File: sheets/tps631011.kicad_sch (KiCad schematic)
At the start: 4 parts, among them U2 XC6220B331ER-G

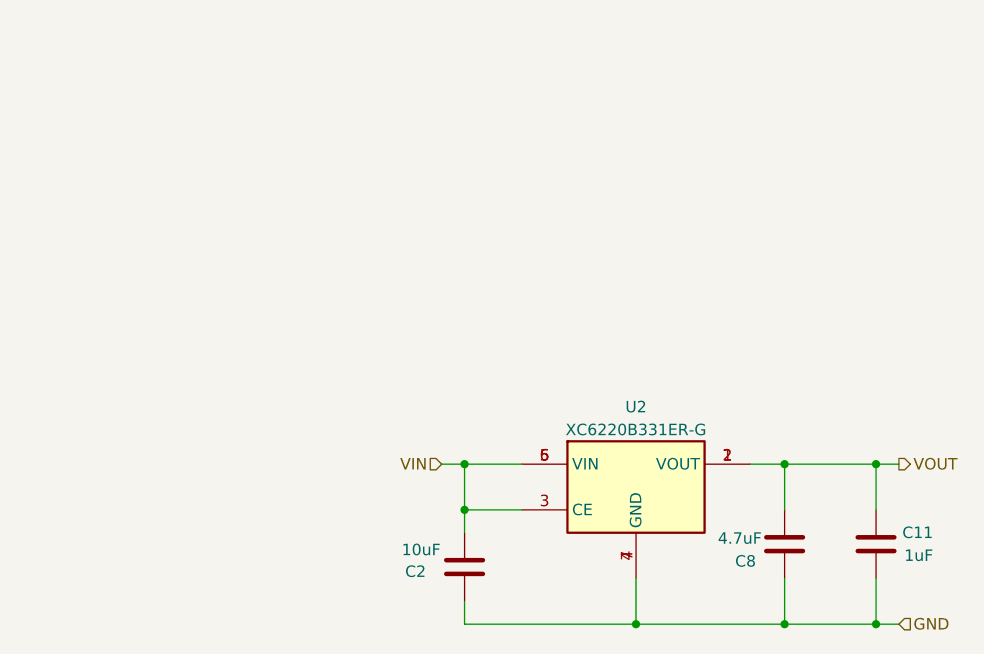
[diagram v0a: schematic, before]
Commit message: More cleanup
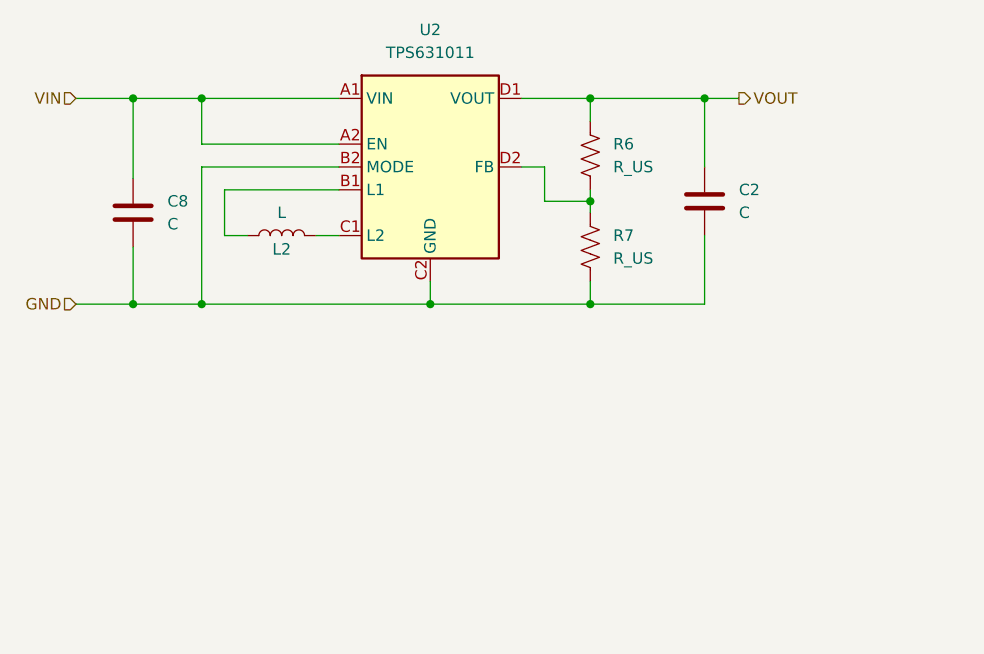
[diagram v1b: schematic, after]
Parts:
- removed C11: 1uF, Capacitor_SMD:C_0402_1005Metric, symbol Device:C
- removed U2: XC6220B331ER-G, PowerFeather:USP-6C_TOR, symbol Regulator_Linear:XC6220B331MR
- added L2: L, symbol Device:L
- added R6, R7: R_US, symbol Device:R_US
- added U2: TPS631011, symbol PowerFeather_KiCAD_Lib:TPS631011
- C2: value 10uF -> C; footprint Capacitor_SMD:C_0603_1608Metric -> (none); Comment 10V, X5R -> (none); MPN 187-CL10A106KP8NNWC -> (none)
- C8: value 4.7uF -> C; footprint Capacitor_SMD:C_0603_1608Metric -> (none); Comment 10V, X5R -> (none); MPN 187-CL10A475KP8NNND -> (none)
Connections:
- net GND: now also C2.2, R7.2, U2.B2 (MODE), U2.C2 (GND); no longer C2.1
- net VIN: now also C8.1, U2.A1 (VIN), U2.A2 (EN); no longer C2.2
- net VOUT: now also C2.1, R6.1, U2.D1 (VOUT); no longer C8.1
- new net: R6.2, R7.1, U2.D2 (FB)
- new net: L2.1, U2.B1 (L1)
- new net: L2.2, U2.C1 (L2)
